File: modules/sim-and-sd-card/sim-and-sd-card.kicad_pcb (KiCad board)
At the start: 2 copper layers, 22 x 25.4 mm, 2 parts

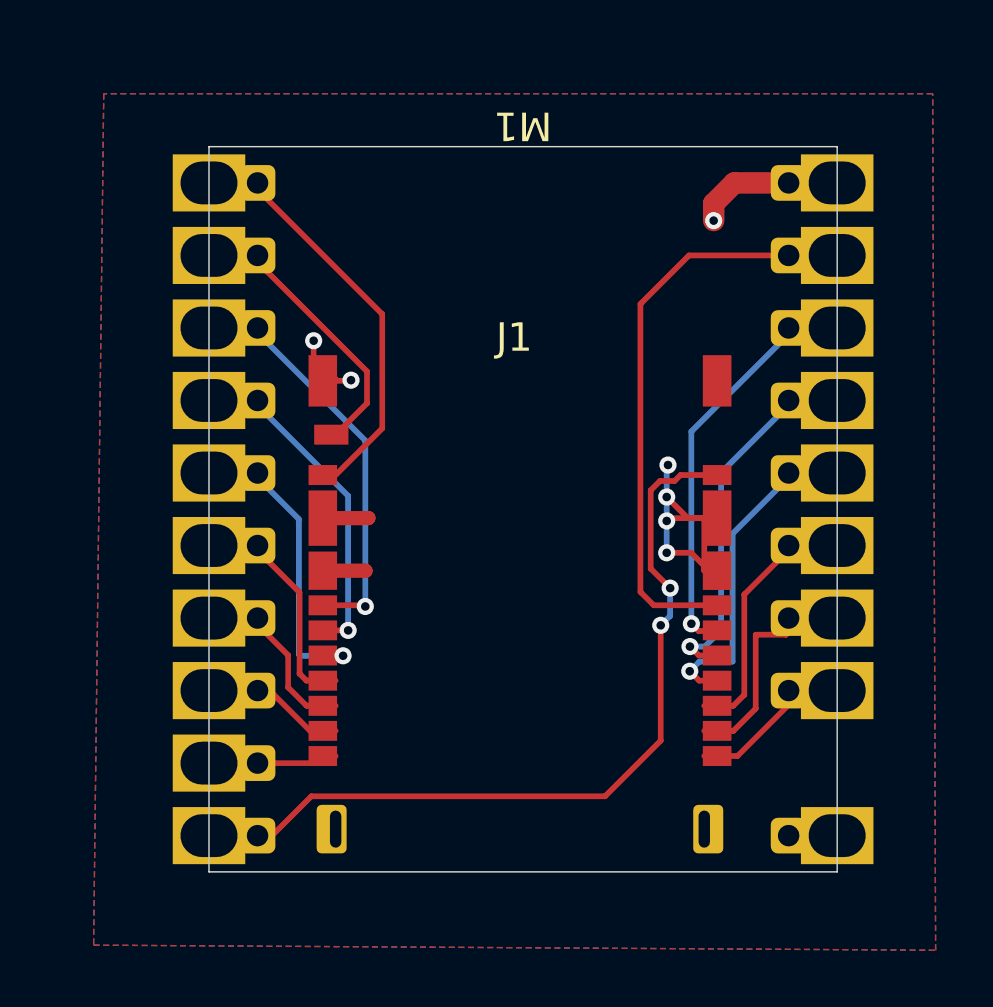
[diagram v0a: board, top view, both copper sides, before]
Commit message: Updating all modules
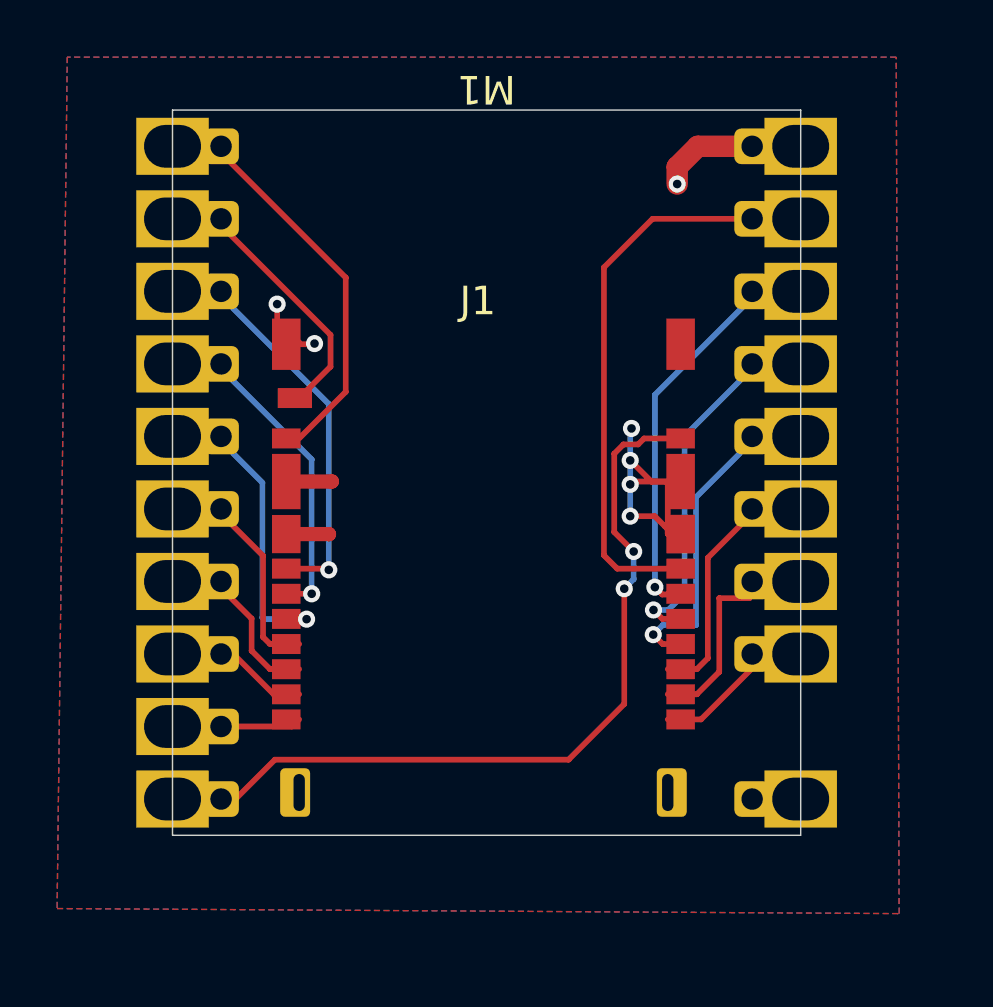
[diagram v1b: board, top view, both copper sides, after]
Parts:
- moved J1 1.81 mm to (58.1, 60.0)
- moved M1 1.81 mm to (58.4, 47.5)
